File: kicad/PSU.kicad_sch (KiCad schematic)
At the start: 60 parts, among them J1 +12V in1, J10 +5V, J11 0V, J2 +12V in2, J3 0v, J4 Conn_02x20_Odd_Even, J5 LED-, J6 LED+, J7 Sw, J8 Sw, J9 +5Vu, Q1 CSD19505, Q2 IRF7319, Q3 CSD19505KCS, U1 LM358, U2 LM22678TJ-ADJ

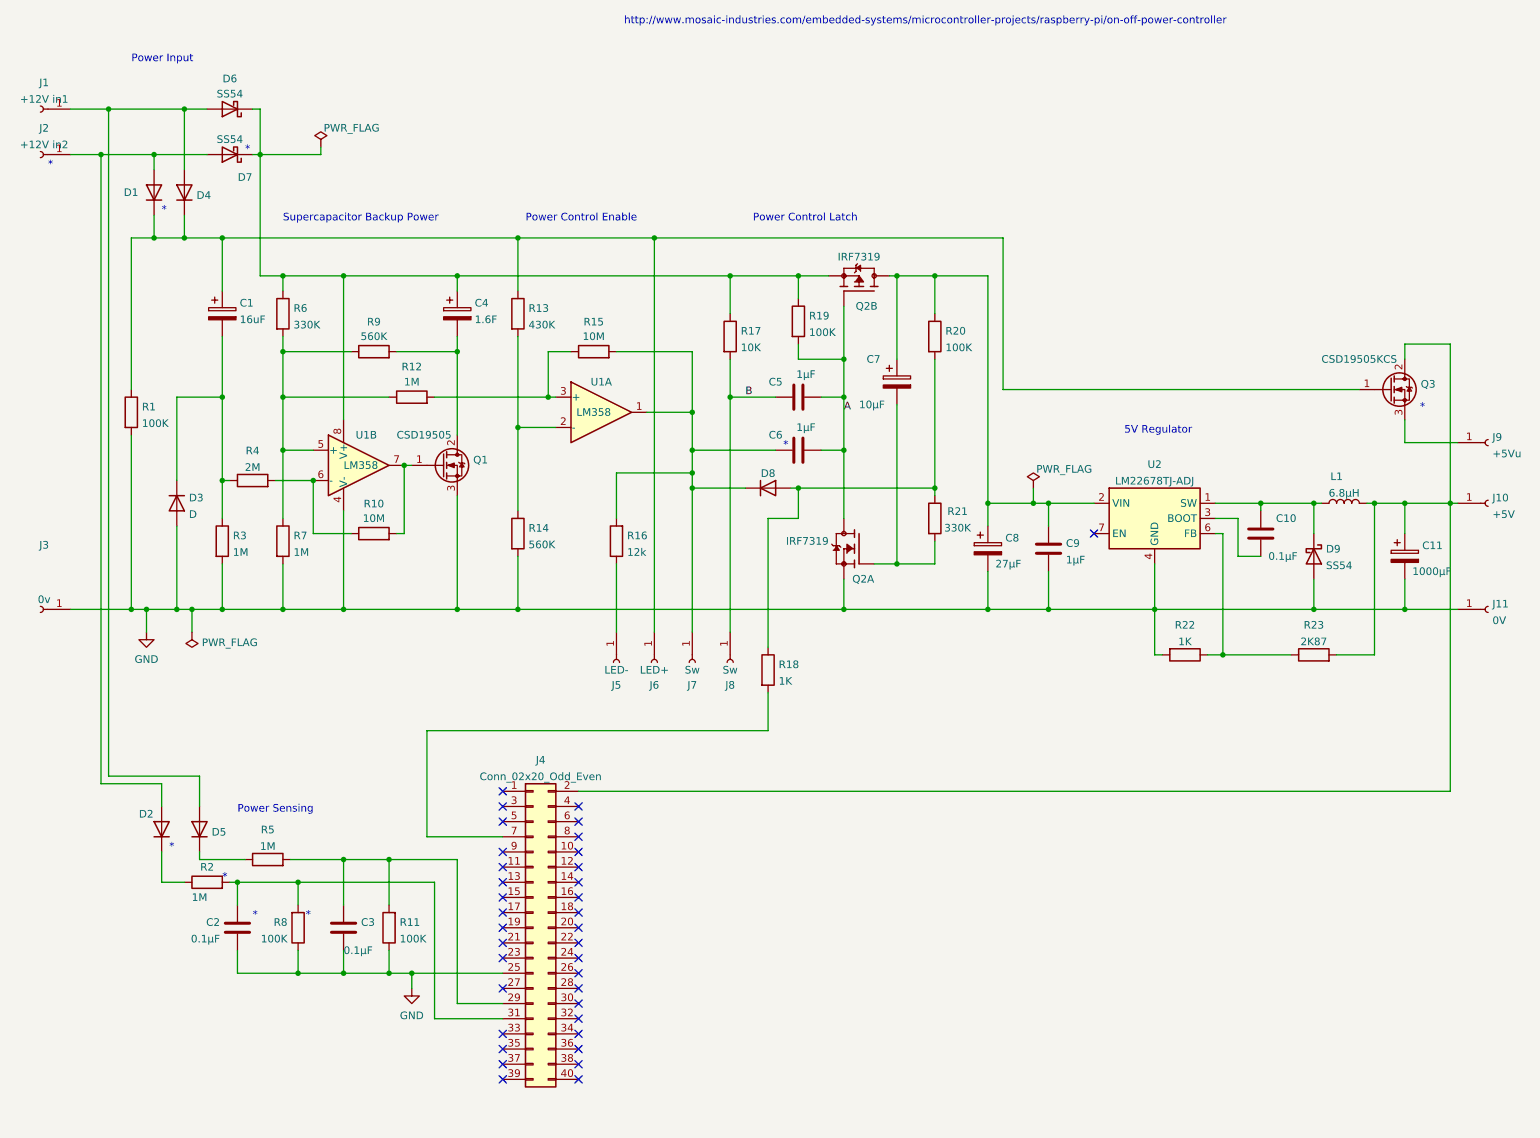
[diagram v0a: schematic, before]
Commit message: Still setting up...
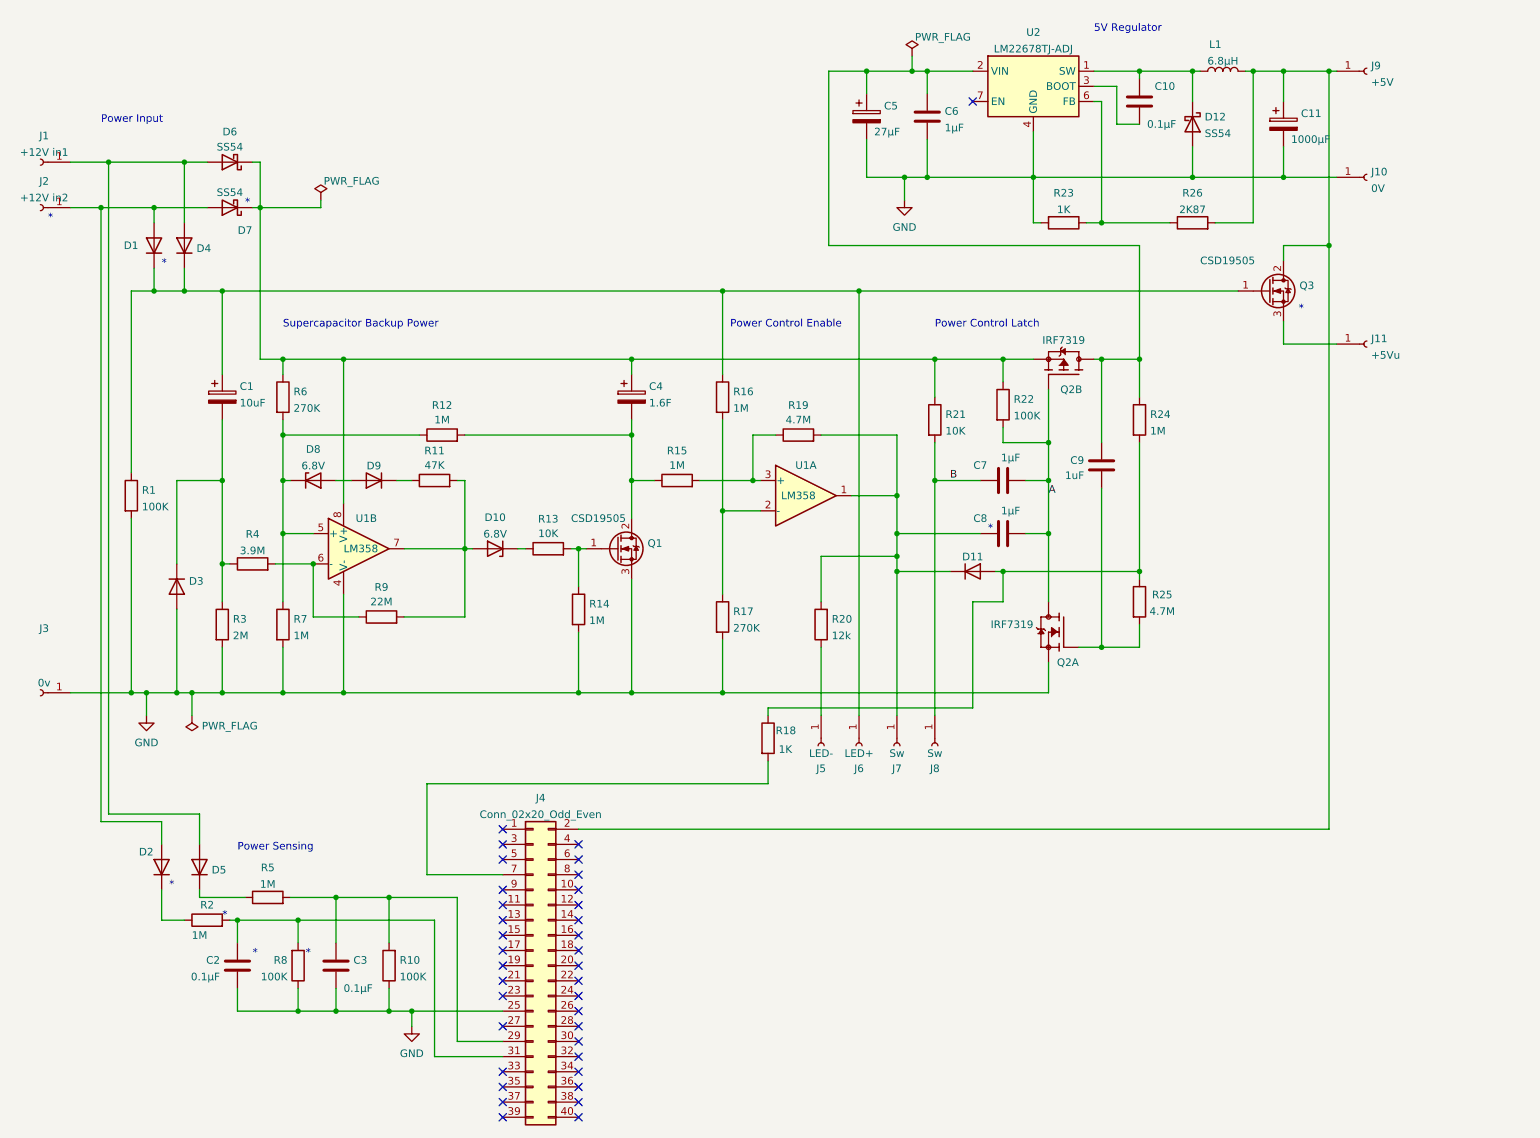
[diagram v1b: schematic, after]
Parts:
- removed C7: 10μF, Capacitor_THT:CP_Radial_D5.0mm_P2.00mm, symbol Device:C_Polarized
- removed R12: 1M, Resistor_THT:R_Axial_DIN0207_L6.3mm_D2.5mm_P10.16mm_Horizontal, symbol Device:R
- added C9: 1uF, Capacitor_THT:C_Disc_D7.5mm_W2.5mm_P5.00mm, symbol Device:C
- added D10, D8: 6.8V, Diode_THT:D_A-405_P7.62mm_Horizontal, symbol Device:D_Zener
- added D9: D, Diode_THT:D_A-405_P7.62mm_Horizontal, symbol Device:D
- added R11: 47K, Resistor_THT:R_Axial_DIN0207_L6.3mm_D2.5mm_P10.16mm_Horizontal, symbol Device:R
- added R13: 10K, Resistor_THT:R_Axial_DIN0207_L6.3mm_D2.5mm_P10.16mm_Horizontal, symbol Device:R
- added R14, R15: 1M, Resistor_THT:R_Axial_DIN0207_L6.3mm_D2.5mm_P10.16mm_Horizontal, symbol Device:R
- C1: value 16uF -> 10uF; footprint Capacitor_THT:CP_Axial_L18.0mm_D6.5mm_P25.00mm_Horizontal -> Capacitor_THT:CP_Radial_D5.0mm_P2.00mm
- Q3: value CSD19505KCS -> CSD19505
- R12: renamed from R9; value 560K -> 1M
- R16: renamed from R13; value 430K -> 1M
- R17: renamed from R14; value 560K -> 270K
- R19: renamed from R15; value 10M -> 4.7M
- R24: renamed from R20; value 100K -> 1M
- R25: renamed from R21; value 330K -> 4.7M
- R3: value 1M -> 2M
- R4: value 2M -> 3.9M
- R6: value 330K -> 270K
- R9: renamed from R10; value 10M -> 22M
- renumbered C8 to C5, C9 to C6, C5 to C7, C6 to C8, D8 to D11, D9 to D12, J11 to J10, J9 to J11, J10 to J9, R11 to R10, R16 to R20, R17 to R21, R19 to R22, R22 to R23, R23 to R26
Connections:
- net GND: now also R14.2
- net at R12.1, R6.2, R7.1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: now also D8.1 (K)
- net at R19.1, U1.3 (+): now also R15.2
- net at Q2.2 (G1), R25.2: now also C9.1
- net at C5.1, C6.1, Q2.5 (D2)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: now also C9.2
- net at C4.2, Q1.2 (D), R12.2: now also R15.1
- net at R9.2, U1.7: now also D10.2 (A), R11.2; no longer Q1.1 (G)
- new net: D9.1 (K), R11.1
- new net: D8.2 (A), D9.2 (A)
- new net: D10.1 (K), R13.1
- new net: Q1.1 (G), R13.2, R14.1
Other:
- note removed: "http://www.mosaic-industries.com/embedded-systems/microcontroller-projects/raspberry-pi/on-off-power-controller"
- company: (none) -> Bloodnok Marine
- moved on the sheet: C1, C10, C11, C2, C3, C4, C5, C6, C7, C8, D1, D11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
